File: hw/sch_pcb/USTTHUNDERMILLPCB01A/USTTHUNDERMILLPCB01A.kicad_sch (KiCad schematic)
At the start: 11 parts, among them U1 ISL21080DIH312Z-TK 1V25, U2 OPA314

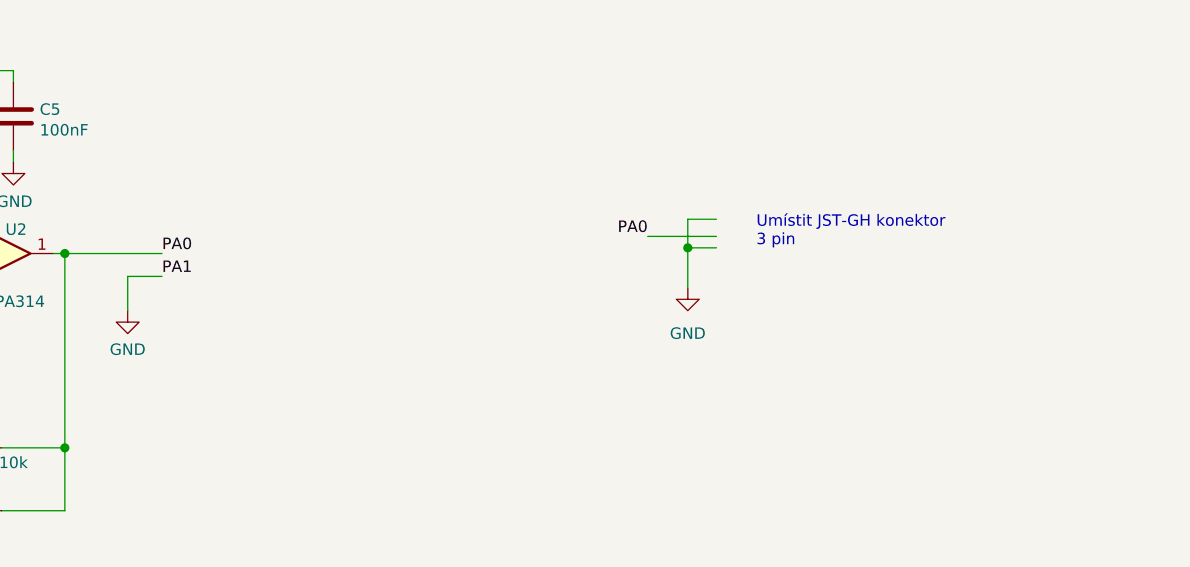
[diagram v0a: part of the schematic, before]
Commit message: Edit PCB
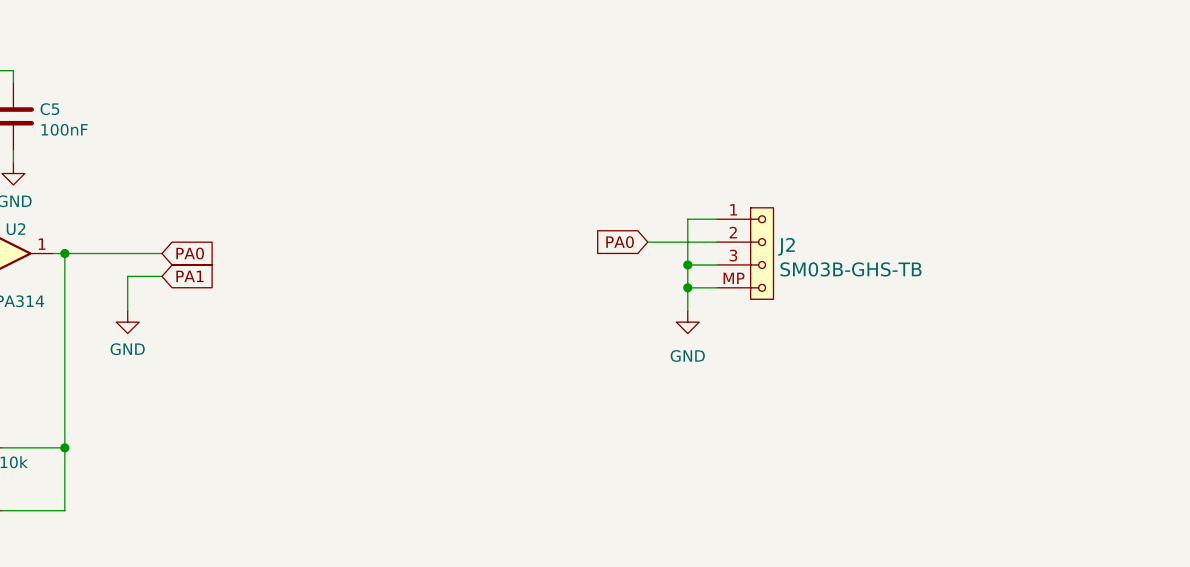
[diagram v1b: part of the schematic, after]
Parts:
- added J2: SM03B-GHS-TB, Connector_JST:JST_GH_SM03B-GHS-TB_1x03-1MP_P1.25mm_Horizontal, symbol MLAB_CONNECTORS_JST:SM03B-GHS-TB
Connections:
- net GND: now also J2.1, J2.3, J2.MP
- net PA0: now also J2.2
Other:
- note removed: "Umístit JST-GH konektor 3 pin"
